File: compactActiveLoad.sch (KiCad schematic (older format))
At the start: 10 parts, among them CON1 Keystone_3002, CON2 Keystone_3002, CON3 LOAD, CON4 +12V, CON5 MOD, Q1 IRLR024NPBF, Q2 IRLR024NPBF, SW1 SW_1290F1123, SW2 SW_1290F1123, U1 Heatsink_55mm_CG128

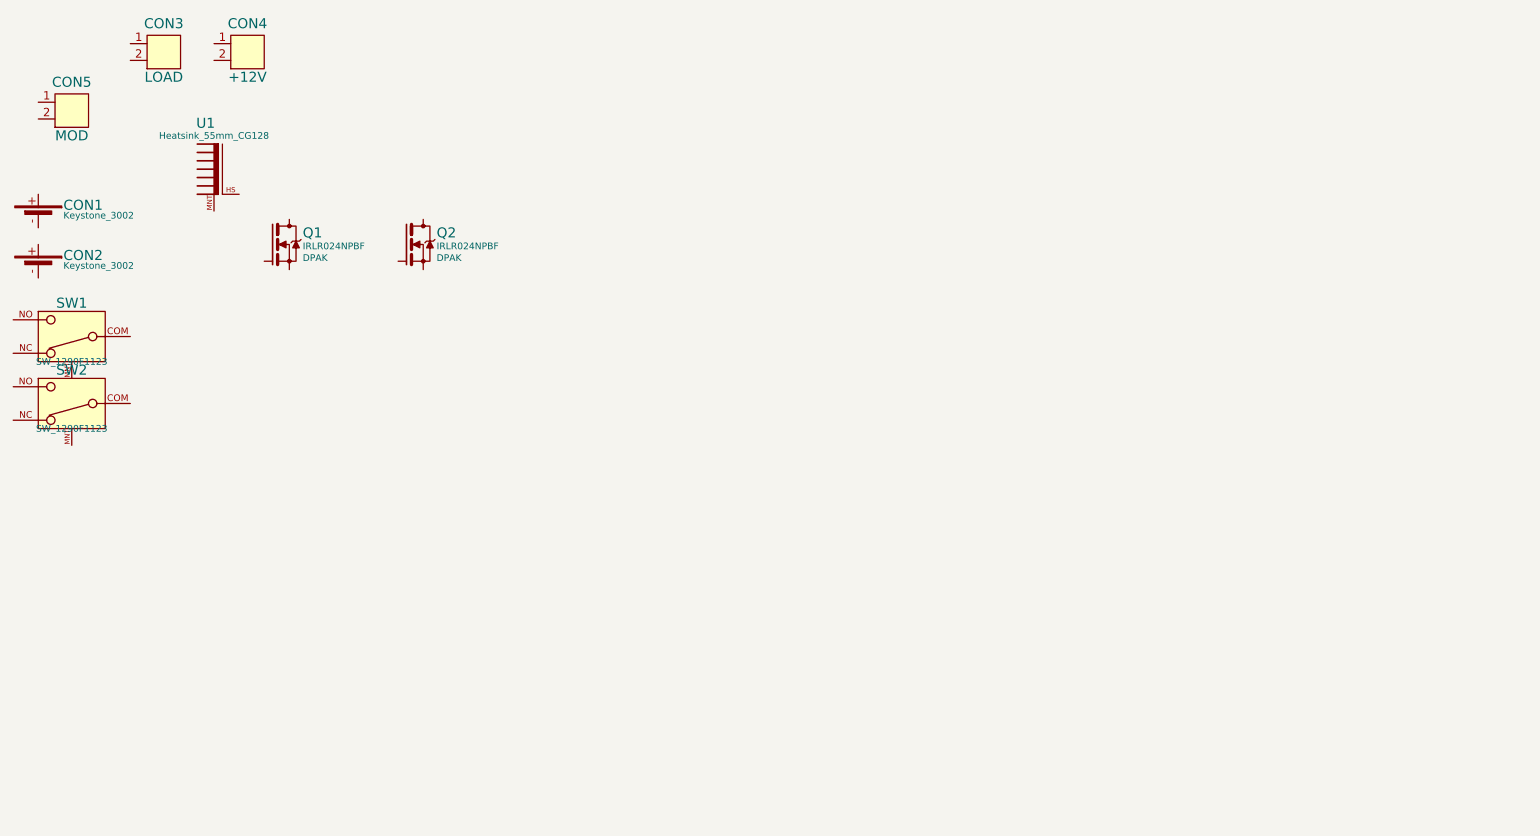
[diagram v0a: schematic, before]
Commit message: Placement
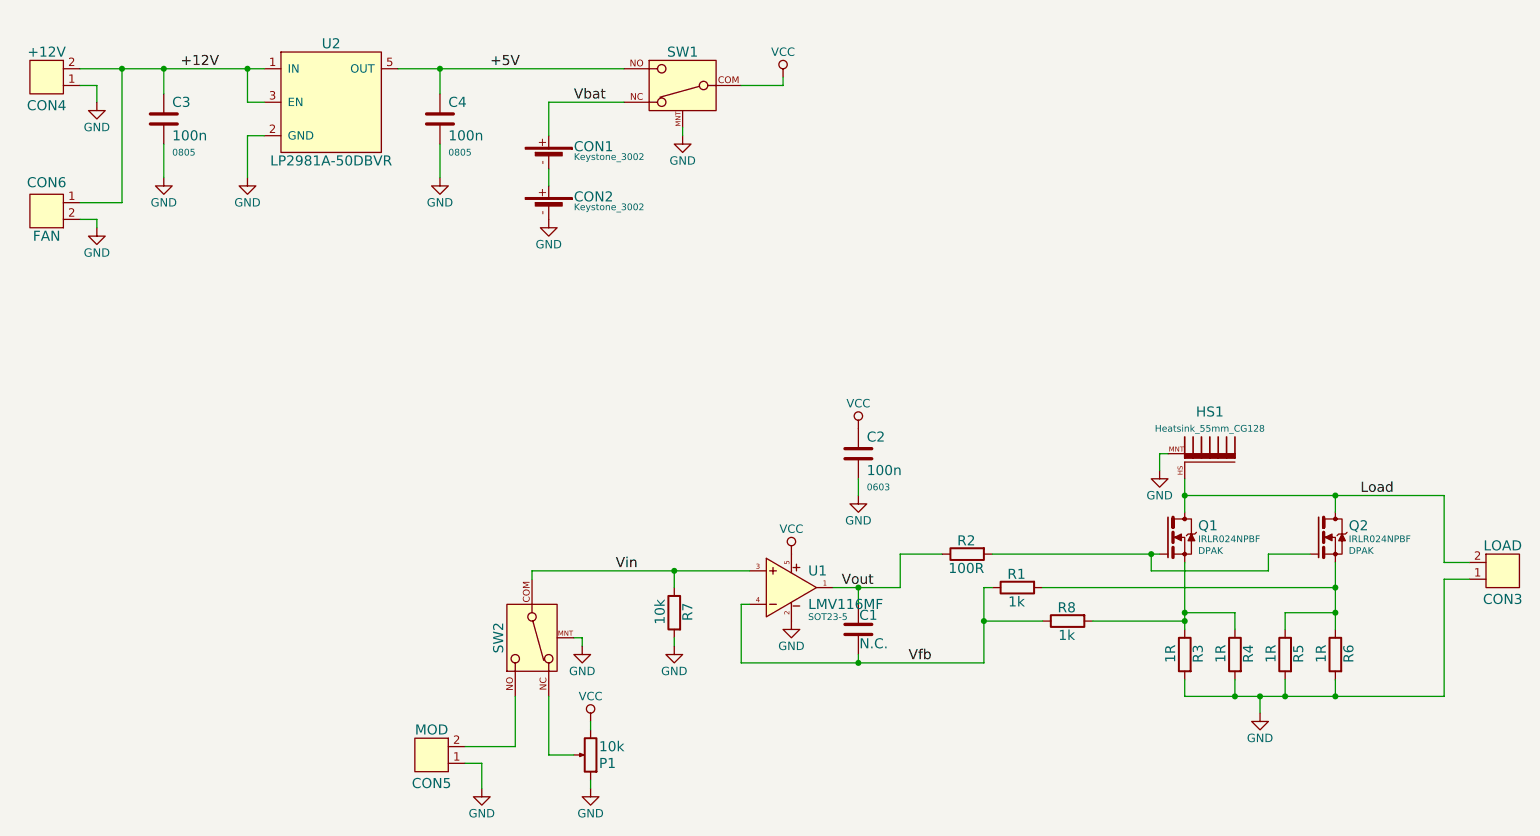
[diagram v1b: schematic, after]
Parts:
- added C1: N.C., pnRLC:0603, symbol C
- added C2: 100n, 0603, symbol C
- added C3, C4: 100n, 0805, symbol C
- added CON6: FAN, pnConnector:PAD2_2x3, symbol CON2
- added P1: 10k, pnRLC:pot_ACP_CA6VSMD+6001, symbol pot_ACP_CA6VSMD+6001
- added R1, R8: 1k, pnRLC:0603, symbol R
- added R2: 100R, pnRLC:0603, symbol R
- added R3, R4, R5, R6: 1R, pnRLC:R2010, symbol R
- added R7: 10k, pnRLC:0603, symbol R
- added U1: LMV116MF, SOT23-5, symbol LMV116MF
- added U2: LP2981A-50DBVR, pnSemiconductor:SOT23-5, symbol LP2981A-50DBVR
- renumbered U1 to HS1
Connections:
- net at Q1.1 (G): now also Q2.1 (G), R2.1
- net at Q1.3 (S): now also R3.2, R4.2, R8.1
- net Load: now reaches Q1.4 (D)
- net Load: now also CON3.2, HS1.HS, Q2.4 (D)
- net at Q2.3 (S): now also R1.1, R5.2, R6.2
- net Vbat: now reaches CON1.+
- net Vbat: now also SW1.NC
- net at CON1.-: now also CON2.+
- net GND: now reaches CON2.-
- net GND: now also CON3.1, CON4.1, CON5.1, HS1.MNT, SW1.MNT, SW2.MNT, C2.2, C3.2, C4.2, CON6.2, P1.1, R3.1, R4.1, R5.1, R6.1, R7.1, U1.2 (VSS), U2.2 (GND)
- net VCC: now reaches SW1.COM
- net VCC: now also C2.1, P1.3, U1.5 (VDD)
- net +5V: now reaches SW1.NO
- net +5V: now also C4.1, U2.5 (OUT)
- net Vin: now reaches SW2.COM
- net Vin: now also R7.2, U1.3 (+)
- net at SW2.NC: now also P1.2
- net at SW2.NO: now also CON5.2
- net +12V: now reaches CON4.2
- net +12V: now also C3.1, CON6.1, U2.1 (IN), U2.3 (EN)
- new net Vfb: C1.2, R1.2, R8.2, U1.4 (-)
- new net Vout: C1.1, R2.2, U1.1 (OUT)
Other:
- moved on the sheet: CON1, CON2, CON3, CON4, CON5, HS1, Q1, Q2, SW1, SW2
